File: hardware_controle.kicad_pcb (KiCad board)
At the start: 4 copper layers, 77 x 78 mm, 21 parts, among them J10 JP LED, J7 FB TRANCA, J8 Con. Placa Aux., J9 Con. Alimentação 9.5V, U2 NE555P

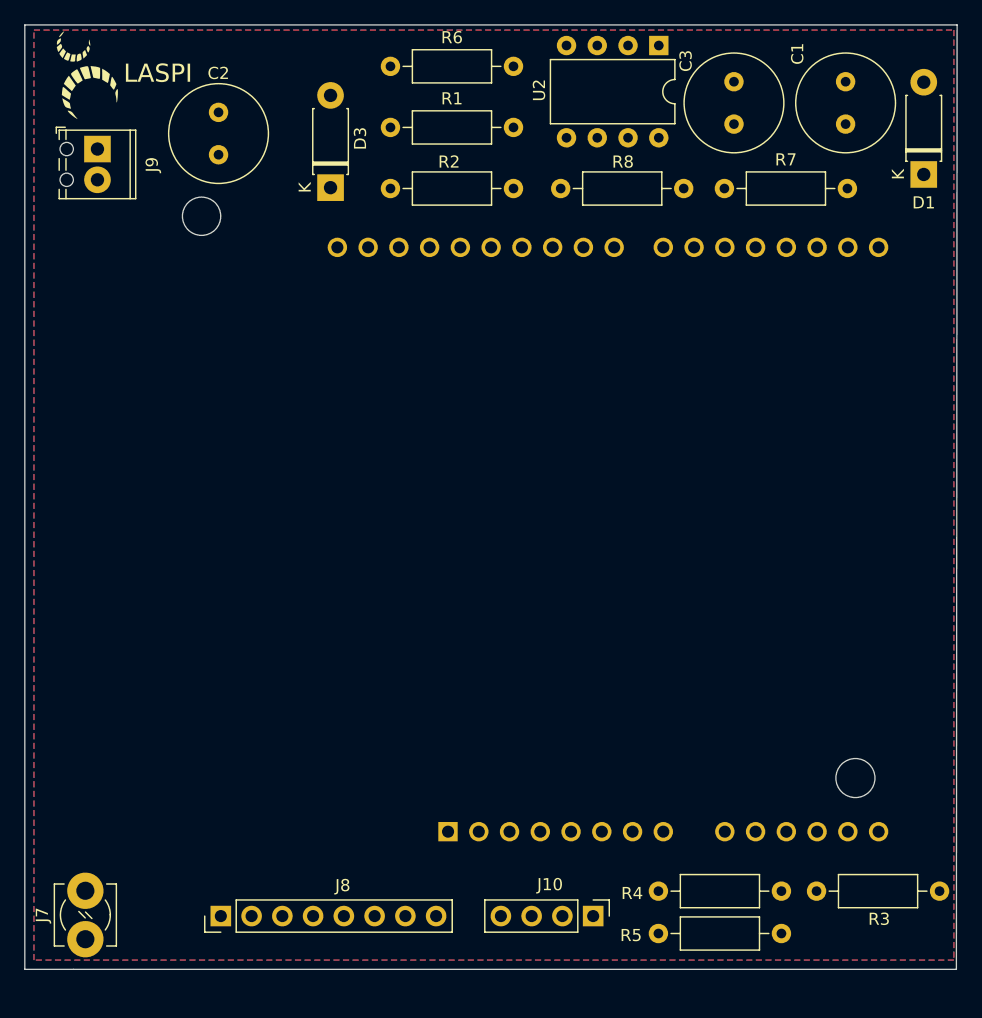
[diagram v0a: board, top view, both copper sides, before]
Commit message: Add files via upload
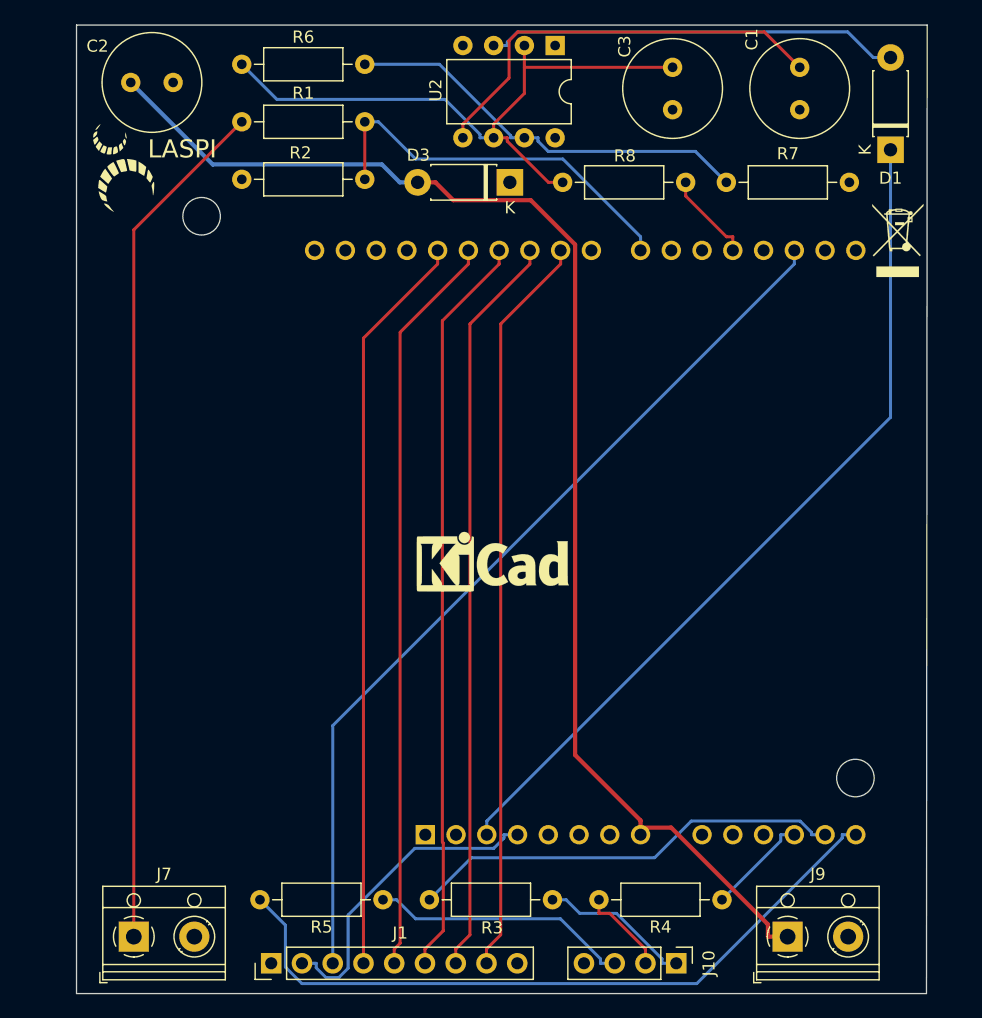
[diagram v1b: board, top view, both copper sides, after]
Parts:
- removed J8: Con. Placa Aux., Connector_PinHeader_2.54mm:PinHeader_1x08_P2.54mm_Vertical
- added J1: Con. Placa Aux., Connector_PinHeader_2.54mm:PinHeader_1x09_P2.54mm_Vertical, F.Cu at (105.3, 113.5)
- added REF**: WEEE-Logo_4.2x6mm_SilkScreen, Symbol:WEEE-Logo_4.2x6mm_SilkScreen, F.Cu at (157.1, 53.8)
- J7: footprint TerminalBlock_MetzConnect:TerminalBlock_MetzConnect_360381_1x01_Horizontal_ScrewM3.0 -> TerminalBlock_RND:TerminalBlock_RND_205-00012_1x02_P5.00mm_Horizontal
- J9: footprint TerminalBlock_Phoenix:TerminalBlock_Phoenix_MPT-0,5-2-2.54_1x02_P2.54mm_Horizontal -> TerminalBlock_RND:TerminalBlock_RND_205-00012_1x02_P5.00mm_Horizontal
- REFe: moved to F.Cu
- moved J9 86.5 mm to (148.0, 111.3), turned to 0 degrees
- moved REFe 50.3 mm to (123.7, 80.8), turned to 0 degrees
- moved R5 33.0 mm to (104.4, 108.2)
- moved R3 32.0 mm to (118.4, 108.2)
- moved D3 14.8 mm to (125.1, 49.0), turned to 180 degrees
- moved R2 12.3 mm to (113.1, 48.8)
- moved R1 12.3 mm to (102.9, 44.0)
- moved R6 12.3 mm to (102.9, 39.2)
- moved U2 8.56 mm to (128.8, 37.7)
- moved logolaspi 8.24 mm to (93.0, 47.8)
- moved J10 7.89 mm to (138.8, 113.5)
- moved C2 7.66 mm to (93.8, 40.8), turned to 0 degrees
- moved C3 5.21 mm to (138.5, 39.5)
- moved R4 4.96 mm to (142.6, 108.2)
- moved J7 4.01 mm to (94.0, 111.3), turned to 0 degrees
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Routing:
- net /+9.5: track 0.00 -> 109.7 mm
- net /TR_CNTRL: track 0.00 -> 74.7 mm
- net Net-(J7-Pad1): track 0.00 -> 71.0 mm
- net /NRESET_MCU: track 0.00 -> 70.4 mm
- net /MOSI: track 0.00 -> 61.5 mm
- net /SCLK: track 0.00 -> 61.4 mm
- net /RST: track 0.00 -> 61.4 mm
- net /MISO: track 0.00 -> 61.4 mm
- net /CE: track 0.00 -> 61.4 mm
- net /vermelho: track 0.00 -> 59.4 mm
- net /R2: track 0.00 -> 51.8 mm
- net /azul: track 0.00 -> 35.9 mm
- net /CV: track 0.00 -> 35.1 mm
- net Net-(D1-Pad2): track 0.00 -> 34.3 mm
- net /R1: track 0.00 -> 34.2 mm
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- added copper zone on In1.Cu, net /+5
- added copper zone on In2.Cu, net GND
- removed copper zone on B.Cu, net /+5
- removed copper zone on F.Cu, net GND
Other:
- board size 77 x 78 mm -> 70.3 x 80 mm

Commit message: Add files via upload
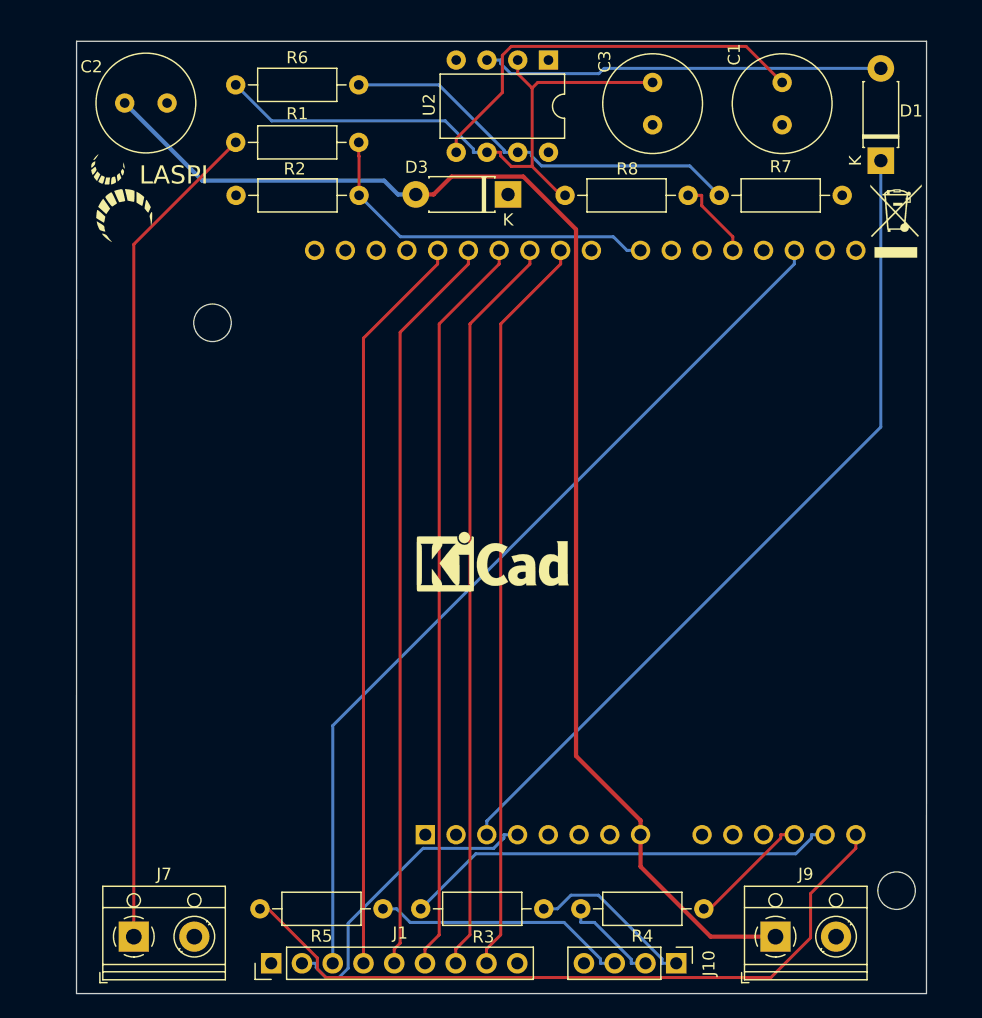
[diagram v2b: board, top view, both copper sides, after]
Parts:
- moved logolaspi 2.49 mm to (92.8, 50.2)
- moved C3 2.07 mm to (136.8, 40.8)
- moved C1 1.91 mm to (147.6, 40.8)
- moved C2 1.77 mm to (93.2, 42.5)
- moved R1 1.77 mm to (102.4, 45.7)
- moved R6 1.77 mm to (102.4, 41.0)
- moved R4 1.68 mm to (141.1, 109.0)
- moved REF** 1.61 mm to (156.9, 52.2)
- moved R2 1.41 mm to (112.6, 50.1)
- moved U2 1.32 mm to (128.2, 38.9)
- moved R7 1.23 mm to (142.3, 50.1)
- moved D1 1.20 mm to (155.7, 47.2)
- moved R8 1.09 mm to (129.6, 50.1)
- moved R3 1.04 mm to (117.7, 109.0)
- moved D3 1.01 mm to (124.9, 50.0)
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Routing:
- net /ver_porta: track 32.6 -> 29.5 mm
- net Net-(J7-Pad1): track 71.0 -> 69.1 mm
- net /verde: track 8.50 -> 10.2 mm
- net /+9.5: track 109.7 -> 111.2 mm
- net /BLUE_OUT: track 12.6 -> 14.0 mm
- net /NRESET_MCU: track 70.4 -> 69.2 mm
- net /R2: track 51.8 -> 50.7 mm
- net Net-(D1-Pad2): track 34.3 -> 33.3 mm
- net /CV: track 35.1 -> 34.2 mm
- net /nDSCHR_CAP: track 7.54 -> 6.73 mm
- net /GREEN_OUT: track 7.36 -> 8.06 mm
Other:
- board size 70.3 x 80 mm -> 70.2 x 78.7 mm
